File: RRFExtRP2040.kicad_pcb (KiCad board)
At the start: 2 copper layers, 80 x 100 mm, 62 parts, among them J1 Screw_Terminal_01x02, J2 Conn_01x05_Pin, J3 Conn_01x05_Pin, J4 Conn_01x05_Pin, J5 Conn_01x05_Pin, J6 Conn_01x05_Pin, J7 RJ11, SW1 SW_Push, U1 OKI-78SR-5_1.5-W36-C, U2 MCP2518FD-E/SL, U3 MCP2542FD-E/SN, U4 AMS1117-3.3, Y1 40MHz

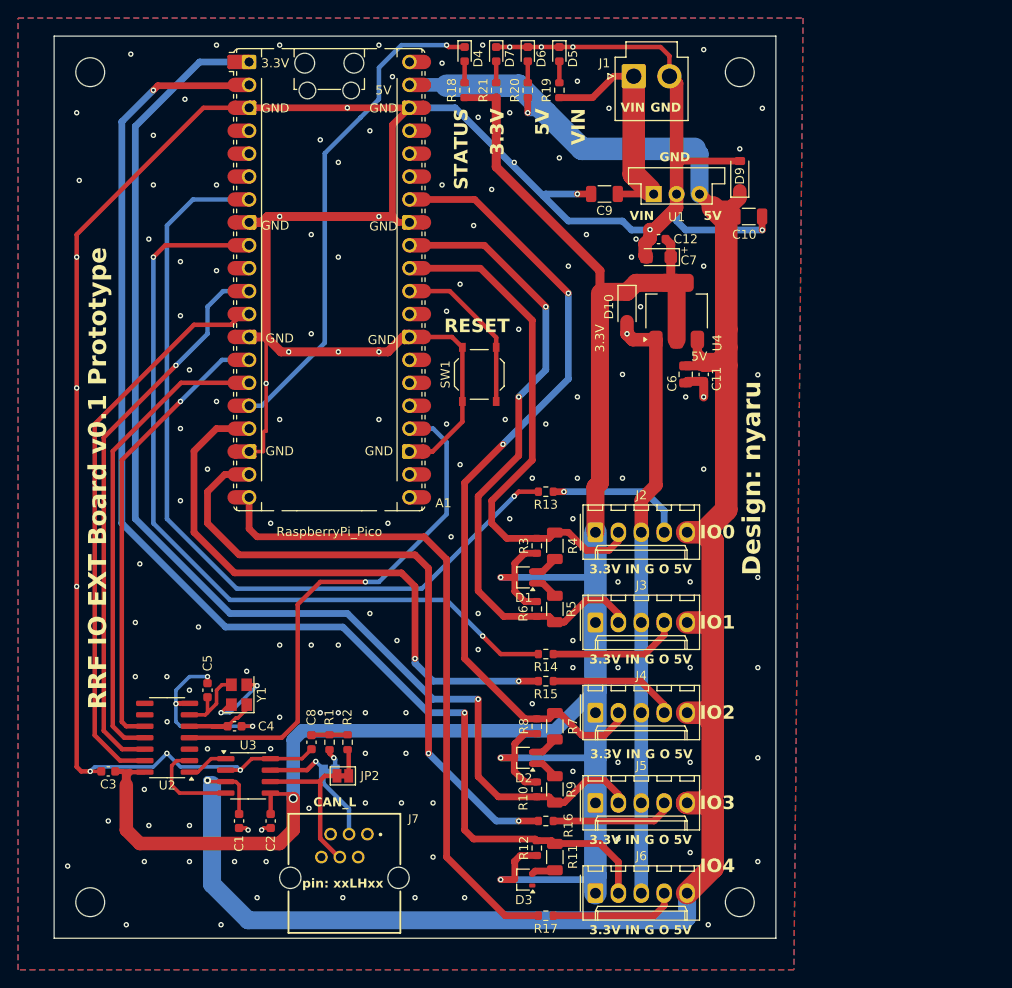
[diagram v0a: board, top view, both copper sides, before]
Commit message: v0.2
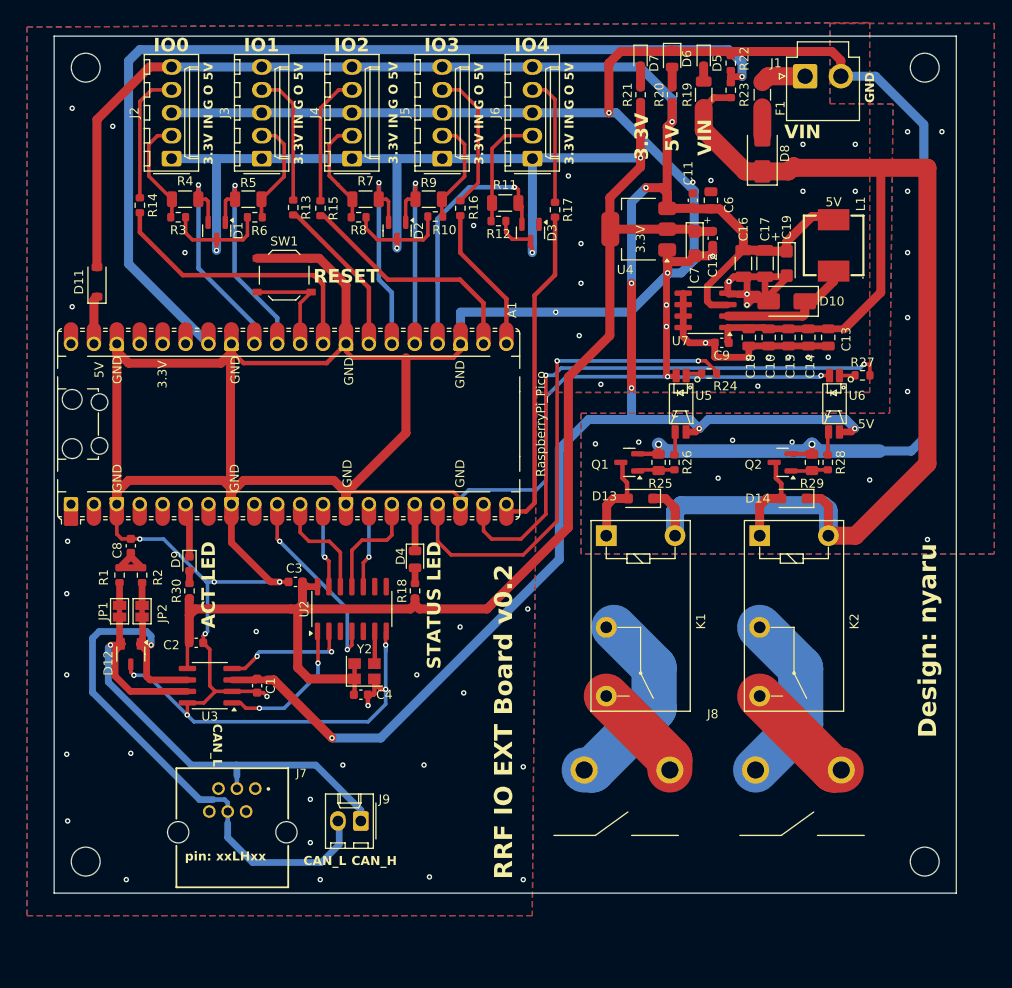
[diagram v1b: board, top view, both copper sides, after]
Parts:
- removed C5: 22pF, Capacitor_SMD:C_0603_1608Metric
- removed REF** (x4): MountingHole_3.2mm_M3, MountingHole:MountingHole_3.2mm_M3
- removed U1: OKI-78SR-5_1.5-W36-C, Converter_DCDC:Converter_DCDC_Murata_OKI-78SR_Vertical
- removed Y1: 40MHz, Crystal:Crystal_SMD_3225-4Pin_3.2x2.5mm
- added C13: 10uF, Capacitor_SMD:C_0805_2012Metric, F.Cu at (155.8, 113.4)
- added C14: 10uF, Capacitor_SMD:C_0805_2012Metric, F.Cu at (153.6, 113.4)
- added C15: 10uF, Capacitor_SMD:C_0805_2012Metric, F.Cu at (151.4, 113.4)
- added C16: 100uF, Capacitor_SMD:C_1206_3216Metric, F.Cu at (146.4, 105.2)
- added C17: 100uF, Capacitor_SMD:C_1206_3216Metric, F.Cu at (148.8, 105.2)
- added C18: 10uF, Capacitor_SMD:C_0805_2012Metric, F.Cu at (147.0, 113.4)
- added C19: 10uF, Capacitor_Tantalum_SMD:CP_EIA-3216-18_Kemet-A, F.Cu at (151.2, 105.2)
- added D11: B5819W, Diode_SMD:D_SOD-123, F.Cu at (74.8, 107.2)
- added D12: ESD2CAN24DBZRQ1, Package_TO_SOT_SMD:SOT-23-3, F.Cu at (78.5, 148.5)
- added D13: SM4007, Diode_SMD:D_SOD-123F, F.Cu at (135.0, 131.2)
- added D14: SM4007, Diode_SMD:D_SOD-123F, F.Cu at (152.0, 131.2)
- added D8: SS34, Diode_SMD:D_SMA, F.Cu at (148.5, 93.0)
- added F1: Fuse 1A, Fuse:Fuse_1206_3216Metric, F.Cu at (148.5, 86.5)
- added H1: MountingHole, MountingHole:MountingHole_3.2mm_M3, F.Cu at (166.5, 83.5)
- added H2: MountingHole, MountingHole:MountingHole_3.2mm_M3, F.Cu at (73.5, 83.5)
- added H3: MountingHole, MountingHole:MountingHole_3.2mm_M3, F.Cu at (166.5, 171.5)
- added H4: MountingHole, MountingHole:MountingHole_3.2mm_M3, F.Cu at (73.5, 171.5)
- added J8: Screw_Terminal_01x04, Library:HB9500-9.5-4P, F.Cu at (143.0, 165.2)
- added J9: Conn_01x02_Pin, Connector_Molex:Molex_KK-254_AE-6410-02A_1x02_P2.54mm_Vertical, F.Cu at (104.0, 167.0)
- added K1: G5Q-EL3-DC24V, Relay_THT:Relay_SPST_Omron-G5Q-1A, F.Cu at (131.2, 135.4)
- added K2: G5Q-EL3-DC24V, Relay_THT:Relay_SPST_Omron-G5Q-1A, F.Cu at (148.2, 135.4)
- added L1: 68uh, Library:IND-SMD_L7.2-W6.6_GPSR07X0, F.Cu at (156.4, 103.2)
- added Q1: AO3400A, Package_TO_SOT_SMD:SOT-23, F.Cu at (133.8, 127.2)
- added Q2: AO3400A, Package_TO_SOT_SMD:SOT-23, F.Cu at (150.8, 127.2)
- added R22: 4K7, Resistor_SMD:R_0603_1608Metric, F.Cu at (145.0, 83.0)
- added R23: 47K, Resistor_SMD:R_0603_1608Metric, F.Cu at (145.0, 86.0)
- added R24: 390R, Resistor_SMD:R_0603_1608Metric, F.Cu at (142.6, 117.4)
- added R25: 10K, Resistor_SMD:R_0805_2012Metric, F.Cu at (137.0, 127.2)
- added R26: 2.2K, Resistor_SMD:R_0603_1608Metric, F.Cu at (138.8, 127.2)
- added R27: 390R, Resistor_SMD:R_0603_1608Metric, F.Cu at (159.6, 117.6)
- added R28: 2.2K, Resistor_SMD:R_0603_1608Metric, F.Cu at (155.8, 127.2)
- added R29: 10K, Resistor_SMD:R_0805_2012Metric, F.Cu at (154.0, 127.2)
- added R30: 4K7, Resistor_SMD:R_0603_1608Metric, F.Cu at (85.0, 141.5)
- added U5: LTV-217, Library:LTV217, F.Cu at (139.5, 120.8)
- added U6: LTV-217, Library:LTV217, F.Cu at (156.5, 120.8)
- added U7: XL1509-5.0, Package_SO:SOIC-8_3.9x4.9mm_P1.27mm, F.Cu at (142.2, 110.4)
- added Y2: YSO110TR, Crystal:Crystal_SMD_3225-4Pin_3.2x2.5mm, F.Cu at (104.4, 150.4)
- C10: footprint Capacitor_SMD:C_1206_3216Metric -> Capacitor_SMD:C_0805_2012Metric
- C4: value 22pF -> 100nF
- C9: value 10uF -> 100nF; footprint Capacitor_SMD:C_1206_3216Metric -> Capacitor_SMD:C_0603_1608Metric
- D1, D2, D3: footprint Package_TO_SOT_SMD:SOT-323_SC-70 -> Package_TO_SOT_SMD:SOT-23
- D10: value ESD 3.3V -> SS34; footprint Diode_SMD:D_SOD-123 -> Diode_SMD:D_SMA
- D4, D6: footprint LED_SMD:LED_0603_1608Metric -> LED_SMD:LED_0805_2012Metric
- D9: value ESD 5V -> LED; footprint Diode_SMD:D_SOD-123 -> LED_SMD:LED_0603_1608Metric
- J1: value Screw_Terminal_01x02 -> Conn_01x02_Pin
- JP1: moved to F.Cu
- R11, R4, R5, R7, R9: value 10K 0.25W -> 4K7 0.25W
- R19: value 5K1 -> 10K; footprint Resistor_SMD:R_0603_1608Metric -> Resistor_SMD:R_1206_3216Metric
- R21: value 200 -> 390R
- moved J6 81.7 mm to (123.0, 93.6), turned to 90 degrees
- moved R17 78.3 mm to (125.5, 99.2), turned to -90 degrees
- moved D9 74.6 mm to (85.0, 138.5), turned to -90 degrees
- moved J5 73.4 mm to (113.0, 93.6), turned to 90 degrees
- moved R11 72.7 mm to (120.0, 98.5), turned to 180 degrees
- moved D3 71.7 mm to (122.8, 101.8), turned to -90 degrees
- moved R12 69.6 mm to (119.2, 100.5), turned to 180 degrees
- moved R16 68.6 mm to (115.0, 99.1), turned to -90 degrees
- moved J4 67.1 mm to (103.0, 93.6), turned to 90 degrees
- moved R14 67.1 mm to (79.5, 98.8), turned to -90 degrees
- moved R9 66.9 mm to (111.5, 98.1), turned to 0 degrees
- moved R10 64.5 mm to (112.2, 100.0), turned to 0 degrees
- moved J3 63.3 mm to (93.0, 93.6), turned to 90 degrees
- moved J2 62.6 mm to (83.0, 93.6), turned to 90 degrees
- moved R7 62.1 mm to (104.5, 98.1), turned to 180 degrees
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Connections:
- A1 pad 1: IO_3_IN -> unconnected-(A1-GPIO0-Pad1)_1
- A1 pad 10: unconnected-(A1-GPIO7-Pad10)_1 -> MCP_INT
- A1 pad 17: Net-(A1-GPIO13) -> RELAY0_OUT
- A1 pad 19: Net-(A1-GPIO14) -> RELAY1_OUT
- A1 pad 2: IO_4_IN -> unconnected-(A1-GPIO1-Pad2)_1
- A1 pad 21: unconnected-(A1-GPIO16-Pad21) -> Net-(A1-GPIO16)
- A1 pad 22: unconnected-(A1-GPIO17-Pad22) -> Net-(A1-GPIO17)
- A1 pad 24: MCP_INT -> IO_4
- A1 pad 25: unconnected-(A1-GPIO19-Pad25) -> IO_3
- A1 pad 26: unconnected-(A1-GPIO20-Pad26)_1 -> IO_2
- A1 pad 27: unconnected-(A1-GPIO21-Pad27) -> Net-(A1-GPIO21)
- A1 pad 29: unconnected-(A1-GPIO22-Pad29)_1 -> Net-(A1-GPIO22)
- A1 pad 31: IO_0_IN -> IO_1
- A1 pad 32: IO_1_IN -> IO_0
- A1 pad 34: IO_2_IN -> POWER_ADC
- A1 pad 39: 5V_EXT -> Net-(A1-VSYS)
- A1 pad 6: unconnected-(A1-GPIO4-Pad6) -> CAN_ACT_LED
- A1 pad 7: Net-(A1-GPIO5) -> unconnected-(A1-GPIO5-Pad7)
- A1 pad 9: Net-(A1-GPIO6) -> unconnected-(A1-GPIO6-Pad9)_1
- C10 pad 1: 5V_EXT -> V_FUSED
- C4 pad 1: Net-(U2-OSC2) -> 3.3V_EXT
- C9 pad 1: VIN -> V_FUSED
- D10 pad 1: 3.3V_EXT -> Net-(D10-K)
- D9 pad 1: 5V_EXT -> CAN_ACT_LED
- D9 pad 2: GND -> Net-(D9-A)
- R13 pad 1: IO_0_OUT -> IO_1_OUT
- R13 pad 2: Net-(A1-GPIO5) -> Net-(A1-GPIO21)
- R14 pad 1: IO_1_OUT -> IO_0_OUT
- R14 pad 2: Net-(A1-GPIO6) -> Net-(A1-GPIO22)
- R15 pad 2: Net-(A1-GPIO13) -> Net-(A1-GPIO17)
- R16 pad 2: Net-(A1-GPIO14) -> Net-(A1-GPIO16)
- R19 pad 1: VIN -> V_FUSED
- U2 pad 5: Net-(U2-OSC2) -> unconnected-(U2-OSC2-Pad5)
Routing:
- net GND: track 441.9 -> 617.8 mm, vias 157 -> 79
- net V_FUSED: track 0.00 -> 162.2 mm
- net IO_4_IN: track 141.2 -> 13.2 mm, vias 2 -> 0
- net IO_3_IN: track 133.3 -> 12.0 mm, vias 1 -> 0
- net POWER_ADC: track 0.00 -> 110.1 mm, vias 0 -> 1
- net Net-(A1-GPIO5): track 91.6 -> 0.00 mm, vias 1 -> 0
- net Net-(A1-GPIO6): track 88.5 -> 0.00 mm, vias 2 -> 0
- net IO_2_IN: track 89.9 -> 12.1 mm, vias 2 -> 0
- net Net-(A1-GPIO14): track 70.5 -> 0.00 mm, vias 2 -> 0
- net Net-(A1-GPIO13): track 66.1 -> 0.00 mm, vias 2 -> 0
- net RELAY1_OUT: track 0.00 -> 64.4 mm, vias 0 -> 2
- net IO_1_IN: track 71.3 -> 12.0 mm, vias 2 -> 0
- net RELAY0_OUT: track 0.00 -> 55.6 mm, vias 0 -> 2
- net SPI_CS: track 62.6 -> 9.40 mm, vias 0 -> 1
- net SPI_MISO: track 62.5 -> 11.5 mm, vias 1 -> 0
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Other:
- board size 80 x 100 mm -> 100 x 95 mm
- board text added: "ACT LED"
- board text added: "RRF IO EXT Board v0.2"
- board text added: "STATUS LED"
- board text removed: "RRF IO EXT Board v0.1 Prototype"
- board text removed: "STATUS"
